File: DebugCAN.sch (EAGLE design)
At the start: 58 parts, among them J1 8P8C-LED, J2 XT60PW-M, J3 MA04-1, J4 10118192-0001LF, J5 8P8C-LED, J6 8P8C-LED, J7 8P8C-LED, U1 STM32F302C, U2 NCV7351D1E, U3 SI8621AB-B-IS, U4 AP2127N-3.3TRG1, U5 78L05F, U6 TLP291, X1 CSTCE8M00G55

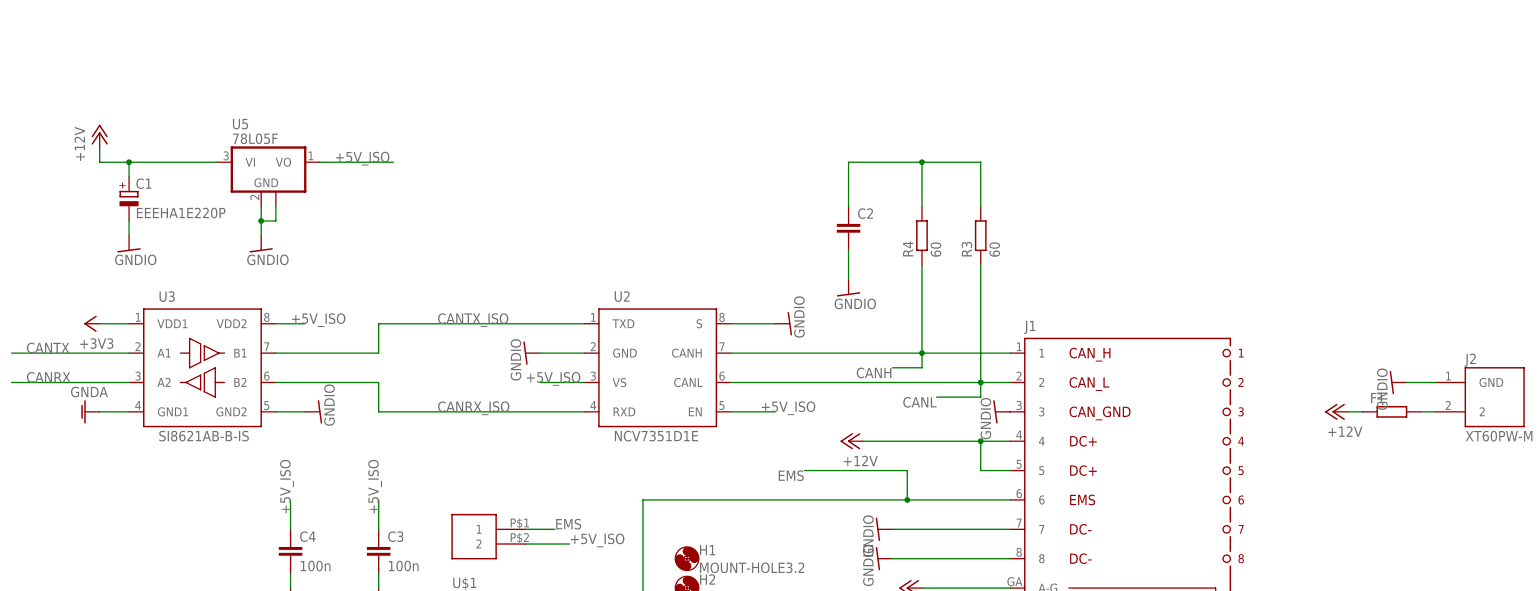
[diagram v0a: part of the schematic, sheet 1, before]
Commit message: change F1
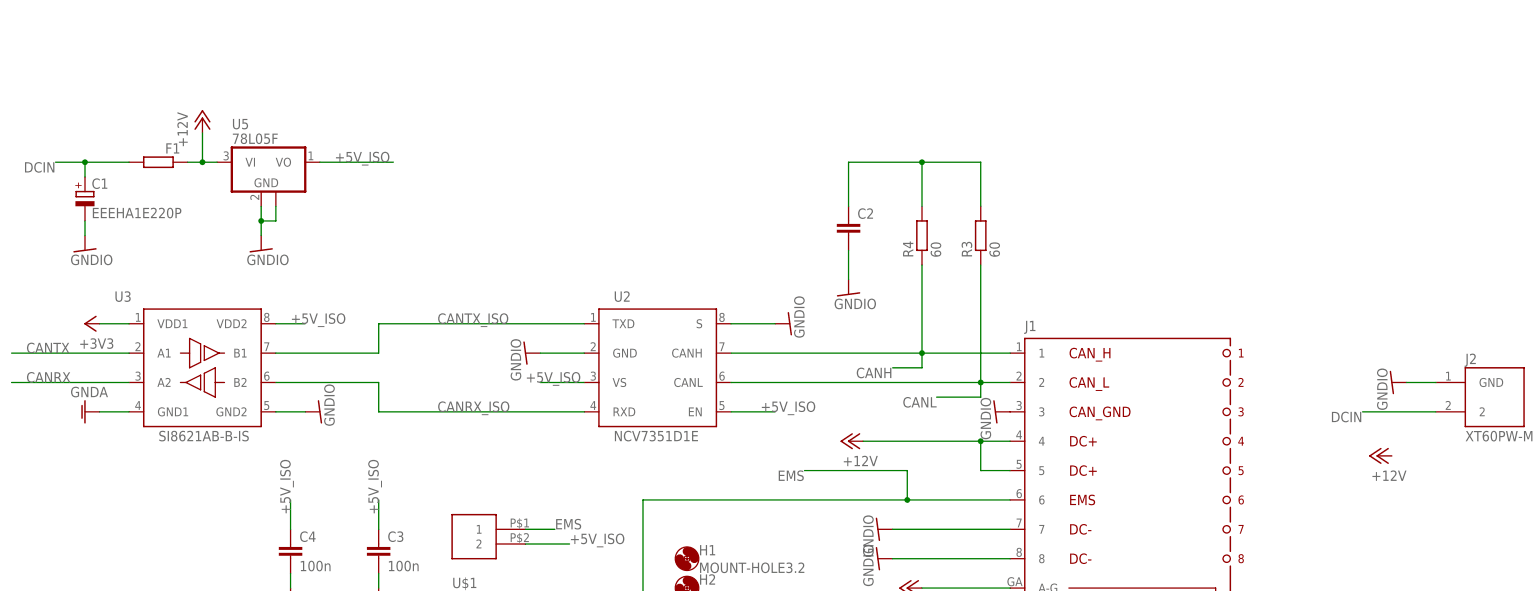
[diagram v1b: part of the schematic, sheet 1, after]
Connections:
- removed net N$1: F1.2, J2.2
- new net DCIN: C1.+, F1.2, J2.2
- net +12V: no longer C1.+
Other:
- moved on the sheet: C1, F1
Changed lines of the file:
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@@
 </instance>
 <instance part="U3" gate="G$1" x="30.48" y="66.04" smashed="yes">
-<attribute name="NAME" x="22.86" y="77.47" size="1.778" layer="95"/>
+<attribute name="NAME" x="15.24" y="77.47" size="1.778" layer="95"/>
 <attribute name="VALUE" x="22.86" y="53.34" size="1.778" layer="96"/>
 </instance>
@@
 <attribute name="VALUE" x="158.242" y="85.09" size="1.778" layer="96" rot="R90"/>
 </instance>
-<instance part="P+1" gate="1" x="12.7" y="106.68" smashed="yes">
-<attribute name="VALUE" x="10.16" y="101.6" size="1.778" layer="96" rot="R90"/>
-</instance>
-<instance part="C1" gate="G$1" x="17.78" y="96.52" smashed="yes">
-<attribute name="NAME" x="18.923" y="97.0026" size="1.778" layer="95"/>
-<attribute name="VALUE" x="18.923" y="91.9226" size="1.778" layer="96"/>
-</instance>
-<instance part="GND9" gate="G$1" x="17.78" y="86.36" smashed="yes">
-<attribute name="VALUE" x="15.24" y="83.82" size="1.778" layer="96"/>
+<instance part="P+1" gate="1" x="30.48" y="109.22" smashed="yes">
+<attribute name="VALUE" x="27.94" y="104.14" size="1.778" layer="96" rot="R90"/>
+</instance>
+<instance part="C1" gate="G$1" x="10.16" y="96.52" smashed="yes">
+<attribute name="NAME" x="11.303" y="97.0026" size="1.778" layer="95"/>
+<attribute name="VALUE" x="11.303" y="91.9226" size="1.778" layer="96"/>
+</instance>
+<instance part="GND9" gate="G$1" x="10.16" y="86.36" smashed="yes">
+<attribute name="VALUE" x="7.62" y="83.82" size="1.778" layer="96"/>
 </instance>
 <instance part="C4" gate="G$1" x="45.72" y="35.56" smashed="yes">
@@
 <attribute name="VALUE" x="233.68" y="66.04" size="1.778" layer="96" rot="R270"/>
 </instance>
-<instance part="P+3" gate="1" x="226.06" y="58.42" smashed="yes" rot="R90">
-<attribute name="VALUE" x="231.14" y="55.88" size="1.778" layer="96" rot="R180"/>
+<instance part="P+3" gate="1" x="233.68" y="50.8" smashed="yes" rot="R90">
+<attribute name="VALUE" x="238.76" y="48.26" size="1.778" layer="96" rot="R180"/>
 </instance>
 <instance part="J2" gate="G$1" x="254" y="60.96" smashed="yes">
@@
 <attribute name="VALUE" x="270.51" y="159.258" size="1.778" layer="96"/>
 </instance>
-<instance part="F1" gate="G$1" x="236.22" y="58.42" smashed="yes">
-<attribute name="NAME" x="232.41" y="59.9186" size="1.778" layer="95"/>
-<attribute name="VALUE" x="232.41" y="55.118" size="1.778" layer="96"/>
+<instance part="F1" gate="G$1" x="22.86" y="101.6" smashed="yes" rot="MR0">
+<attribute name="NAME" x="26.67" y="103.0986" size="1.778" layer="95" rot="MR0"/>
+<attribute name="VALUE" x="26.67" y="98.298" size="1.778" layer="96" rot="MR0"/>
 </instance>
 </instances>
@@
 <pinref part="C1" gate="G$1" pin="-"/>
 <pinref part="GND9" gate="G$1" pin="GNDIO"/>
-<wire x1="17.78" y1="91.44" x2="17.78" y2="88.9" width="0.1524" layer="91"/>
+<wire x1="10.16" y1="91.44" x2="10.16" y2="88.9" width="0.1524" layer="91"/>
 </segment>
 <segment>
@@
 </segment>
 <segment>
-<pinref part="P+1" gate="1" pin="+12V"/>
-<wire x1="33.02" y1="101.6" x2="17.78" y2="101.6" width="0.1524" layer="91"/>
-<wire x1="17.78" y1="101.6" x2="12.7" y2="101.6" width="0.1524" layer="91"/>
-<wire x1="12.7" y1="101.6" x2="12.7" y2="104.14" width="0.1524" layer="91"/>
-<pinref part="C1" gate="G$1" pin="+"/>
-<wire x1="17.78" y1="99.06" x2="17.78" y2="101.6" width="0.1524" layer="91"/>
-<junction x="17.78" y="101.6"/>
-<pinref part="U5" gate="G$1" pin="VI"/>
-</segment>
-<segment>
 <pinref part="P+6" gate="1" pin="+12V"/>
 <pinref part="J5" gate="G$1" pin="4"/>
@@
 <segment>
 <pinref part="F1" gate="G$1" pin="1"/>
-<pinref part="P+3" gate="1" pin="+12V"/>
-<wire x1="231.14" y1="58.42" x2="228.6" y2="58.42" width="0.1524" layer="91"/>
+<pinref part="U5" gate="G$1" pin="VI"/>
+<wire x1="27.94" y1="101.6" x2="30.48" y2="101.6" width="0.1524" layer="91"/>
+<pinref part="P+1" gate="1" pin="+12V"/>
+<wire x1="30.48" y1="101.6" x2="33.02" y2="101.6" width="0.1524" layer="91"/>
+<wire x1="30.48" y1="106.68" x2="30.48" y2="101.6" width="0.1524" layer="91"/>
+<junction x="30.48" y="101.6"/>
 </segment>
 </net>
@@
 </segment>
 </net>
-<net name="N$1" class="0">
+<net name="DCIN" class="2">
+<segment>
+<pinref part="C1" gate="G$1" pin="+"/>
+<wire x1="10.16" y1="99.06" x2="10.16" y2="101.6" width="0.1524" layer="91"/>
+<wire x1="10.16" y1="101.6" x2="5.08" y2="101.6" width="0.1524" layer="91"/>
+<pinref part="F1" gate="G$1" pin="2"/>
+<wire x1="17.78" y1="101.6" x2="10.16" y2="101.6" width="0.1524" layer="91"/>
+<junction x="10.16" y="101.6"/>
+<label x="5.08" y="101.6" size="1.778" layer="95" rot="R180"/>
+</segment>
 <segment>
 <pinref part="J2" gate="G$1" pin="2"/>
-<pinref part="F1" gate="G$1" pin="2"/>
-<wire x1="243.84" y1="58.42" x2="241.3" y2="58.42" width="0.1524" layer="91"/>
-</segment>
-</net>
+<wire x1="243.84" y1="58.42" x2="231.14" y2="58.42" width="0.1524" layer="91"/>
+<label x="231.14" y="58.42" size="1.778" layer="95" rot="R180"/>
+</segment>
+</net>
